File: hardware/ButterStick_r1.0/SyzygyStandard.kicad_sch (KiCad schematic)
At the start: 19 parts, among them J4 SYZYGY-STD, U14 TLV62569DRL

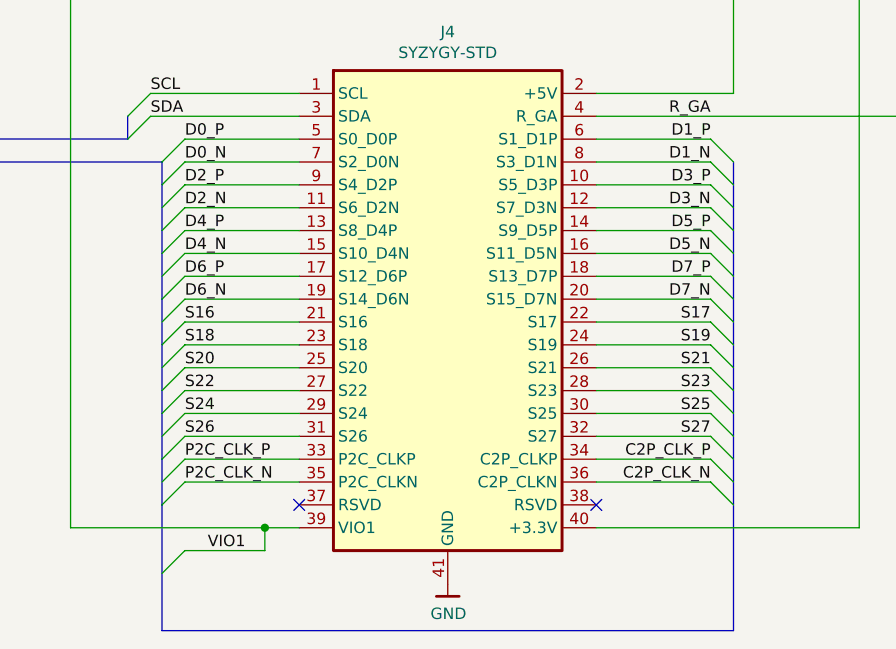
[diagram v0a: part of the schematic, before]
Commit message: hw.r1d0: Review complete, gerbers generated
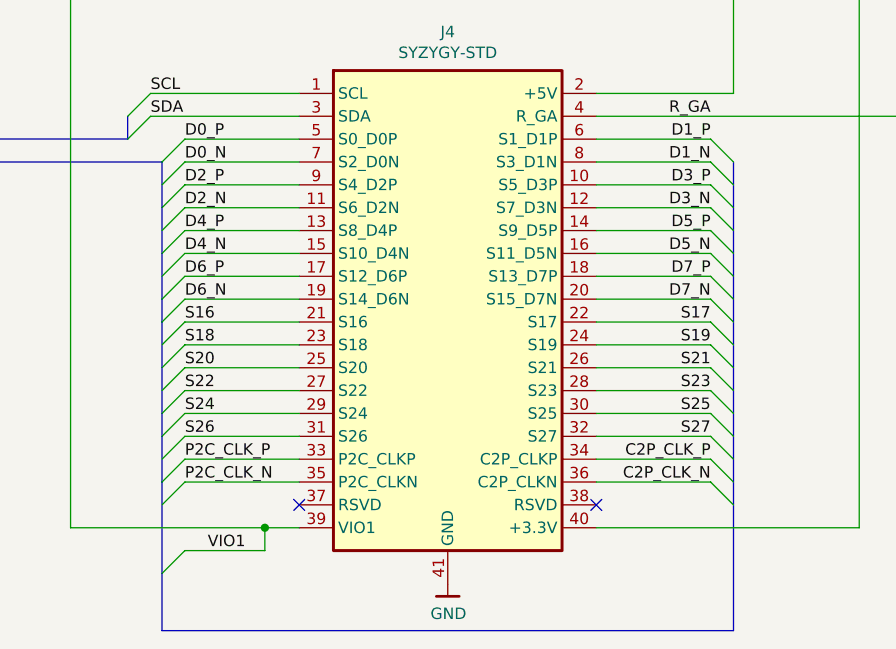
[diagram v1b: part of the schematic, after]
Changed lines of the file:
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@@
 (kicad_sch (version 20200618) (host eeschema "5.99.0-unknown-73168a9~101~ubuntu18.04.1")
-  (page 17 18)
+  (page 16 18)
   (paper "A4")
   (title_block
     (title "ButterStick")
-    (date "2020-07-16")
+    (date "2020-07-17")
     (rev "r1.0")
     (company "GsD")
@@
     (stroke (width 0) (type solid) (color 0 0 0 0))
   )
-  (bus (pts (xy 165.1 101.6) (xy 165.1 104.14))
-    (stroke (width 0) (type solid) (color 0 0 0 0))
-  )
-  (bus (pts (xy 165.1 104.14) (xy 165.1 109.22))
-    (stroke (width 0) (type solid) (color 0 0 0 0))
-  )
-  (bus (pts (xy 165.1 109.22) (xy 165.1 111.76))
+  (bus (pts (xy 165.1 101.6) (xy 165.1 106.68))
+    (stroke (width 0) (type solid) (color 0 0 0 0))
+  )
+  (bus (pts (xy 165.1 106.68) (xy 165.1 111.76))
     (stroke (width 0) (type solid) (color 0 0 0 0))
   )
@@
     (stroke (width 0) (type solid) (color 0 0 0 0))
   )
-  (bus (pts (xy 165.1 116.84) (xy 165.1 121.92))
-    (stroke (width 0) (type solid) (color 0 0 0 0))
-  )
-  (bus (pts (xy 165.1 121.92) (xy 165.1 127))
-    (stroke (width 0) (type solid) (color 0 0 0 0))
-  )
-  (bus (pts (xy 165.1 127) (xy 165.1 129.54))
-    (stroke (width 0) (type solid) (color 0 0 0 0))
-  )
-  (bus (pts (xy 165.1 129.54) (xy 165.1 134.62))
-    (stroke (width 0) (type solid) (color 0 0 0 0))
-  )
-  (bus (pts (xy 165.1 134.62) (xy 165.1 139.7))
-    (stroke (width 0) (type solid) (color 0 0 0 0))
-  )
-  (bus (pts (xy 165.1 139.7) (xy 165.1 153.67))
+  (bus (pts (xy 165.1 116.84) (xy 165.1 119.38))
+    (stroke (width 0) (type solid) (color 0 0 0 0))
+  )
+  (bus (pts (xy 165.1 119.38) (xy 165.1 124.46))
+    (stroke (width 0) (type solid) (color 0 0 0 0))
+  )
+  (bus (pts (xy 165.1 124.46) (xy 165.1 129.54))
+    (stroke (width 0) (type solid) (color 0 0 0 0))
+  )
+  (bus (pts (xy 165.1 129.54) (xy 165.1 132.08))
+    (stroke (width 0) (type solid) (color 0 0 0 0))
+  )
+  (bus (pts (xy 165.1 132.08) (xy 165.1 137.16))
+    (stroke (width 0) (type solid) (color 0 0 0 0))
+  )
+  (bus (pts (xy 165.1 137.16) (xy 165.1 147.32))
+    (stroke (width 0) (type solid) (color 0 0 0 0))
+  )
+  (bus (pts (xy 165.1 147.32) (xy 165.1 153.67))
     (stroke (width 0) (type solid) (color 0 0 0 0))
   )
@@
     (stroke (width 0) (type solid) (color 0 0 0 0))
   )
-  (bus (pts (xy 228.6 127) (xy 228.6 132.08))
-    (stroke (width 0) (type solid) (color 0 0 0 0))
-  )
-  (bus (pts (xy 228.6 132.08) (xy 228.6 137.16))
-    (stroke (width 0) (type solid) (color 0 0 0 0))
-  )
+  (bus (pts (xy 228.6 127) (xy 228.6 129.54))
+    (stroke (width 0) (type solid) (color 0 0 0 0))
+  )
+  (bus (pts (xy 228.6 129.54) (xy 228.6 134.62))
+    (stroke (width 0) (type solid) (color 0 0 0 0))
+  )
+  (bus (pts (xy 228.6 134.62) (xy 228.6 137.16))
+    (stroke (width 0) (type solid) (color 0 0 0 0))
+  )
